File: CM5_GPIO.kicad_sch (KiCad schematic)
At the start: 27 parts, among them J13 THD-02-R, J2 Conn_02x07_Odd_Even, J3 Conn_01x03, J8 THD-20-R, M1 Fan_4pin, M2 Fan_4pin, SW1 Right angle Tact button, U1 TPD4EUSB30, U2 TPD4EUSB30, U3 MagJack-A70-112-331N126, U5 74LVC1G07SE-7

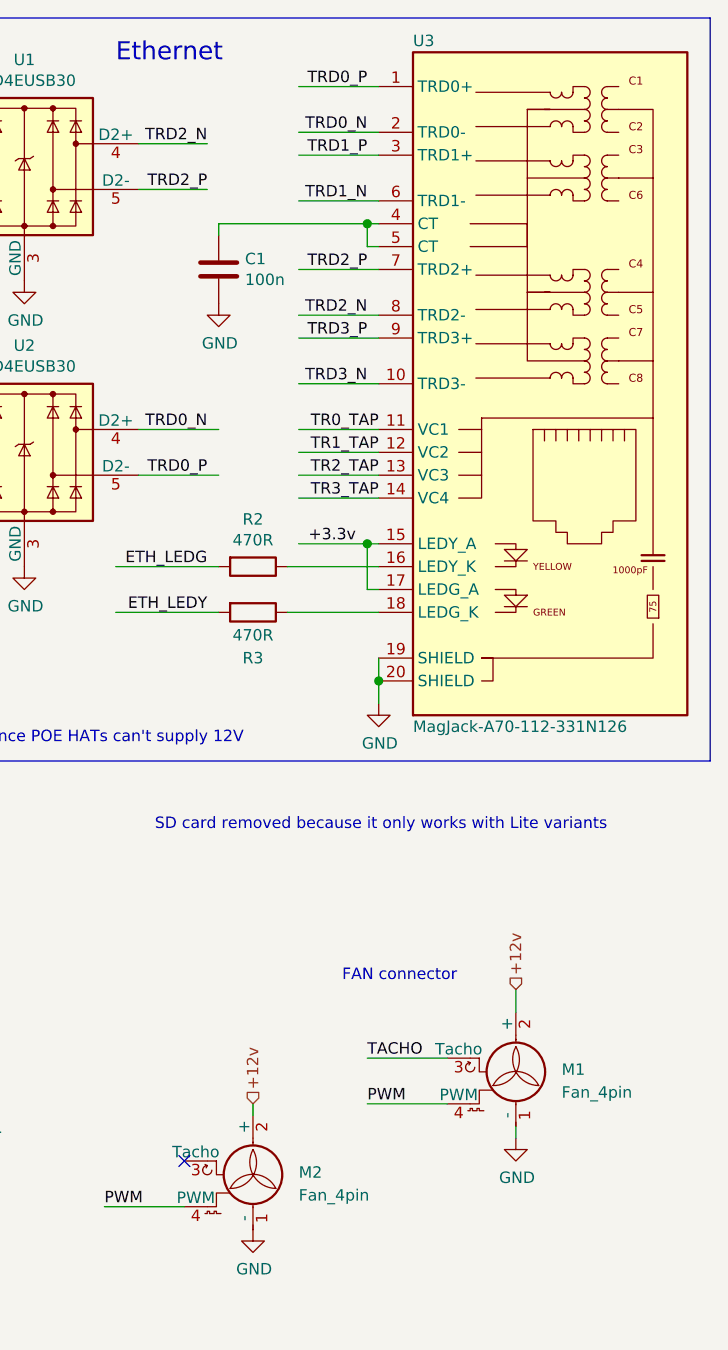
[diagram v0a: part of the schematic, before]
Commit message: update drop in replacements
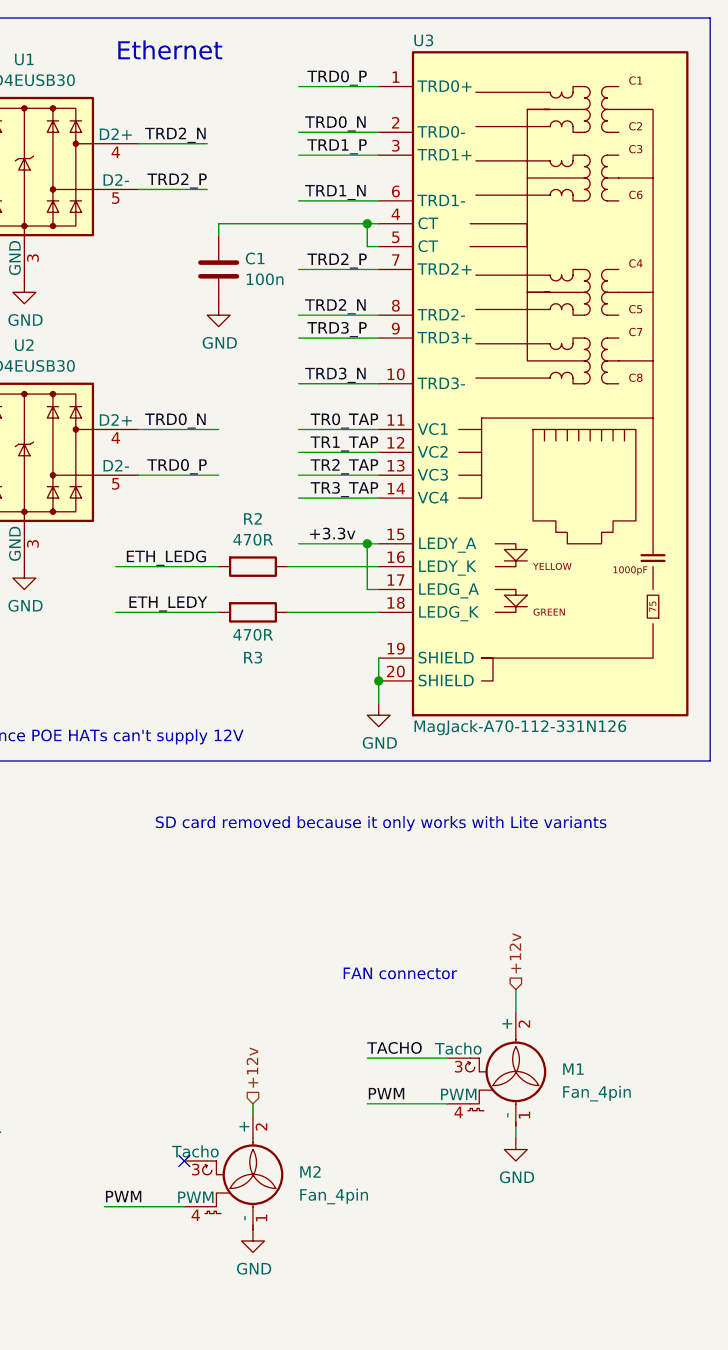
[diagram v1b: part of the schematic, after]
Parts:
- D1: mpn (none) -> 150060RS75000
- D2: mpn (none) -> 150060GS75000
- D3: mpn BAT54-05 -> BAT54C
- J13, J8: mpn (none) -> 61304021121
- J2: mpn (none) -> 61301421121
- SW1: mpn (none) -> 430186050716
- U5: mpn (none) -> 74LVC1G07GW
